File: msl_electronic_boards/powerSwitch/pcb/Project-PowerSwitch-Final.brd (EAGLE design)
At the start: 65.3 x 99.7 mm, 130 parts, among them IC10 BTS6133, IC11 BTS6133, IC12 BTS6133, IC15 BTS6133, IC3 LM2574M-5.0, IC4 BTS555E3146, IC7 MAX202, Q1 16Mhz, T1 BC847, T2 BC849, T5 BC849, T6 BC849, T7 BC849

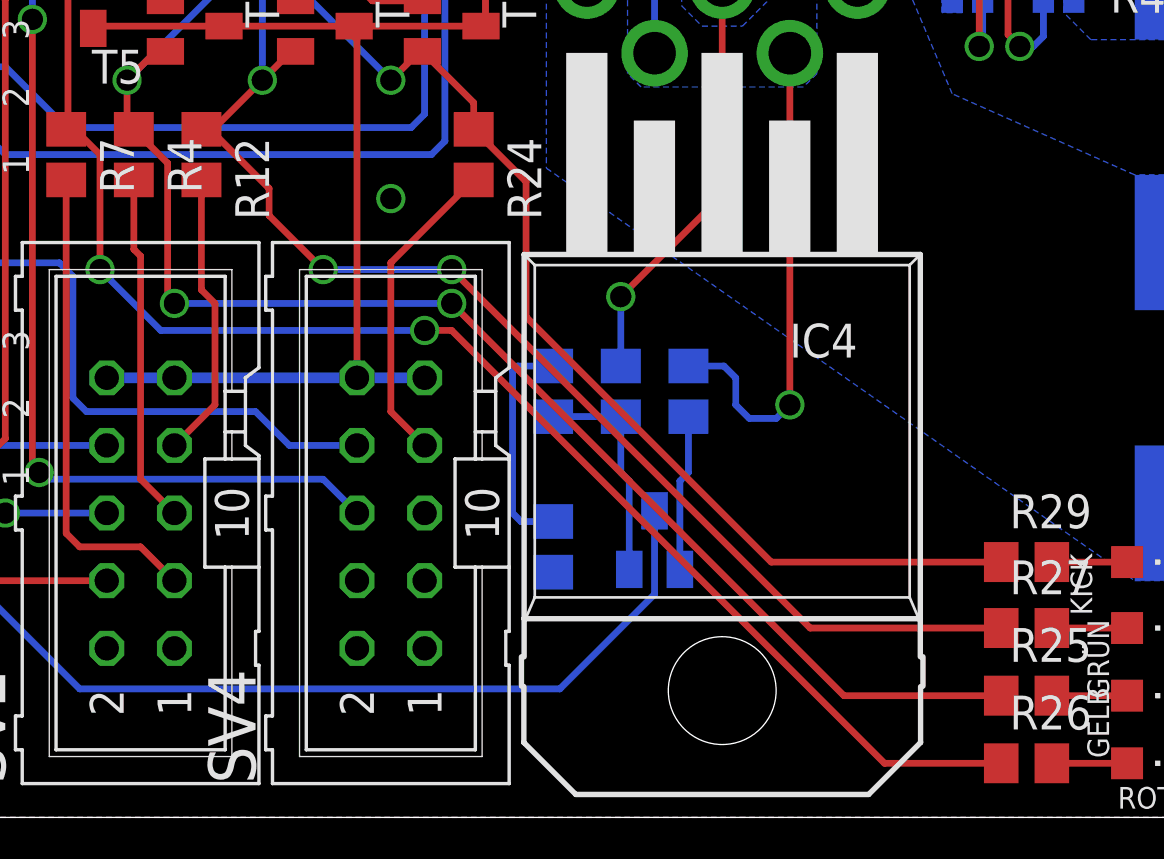
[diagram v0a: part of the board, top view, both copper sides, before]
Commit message: PCB PowerSwitch
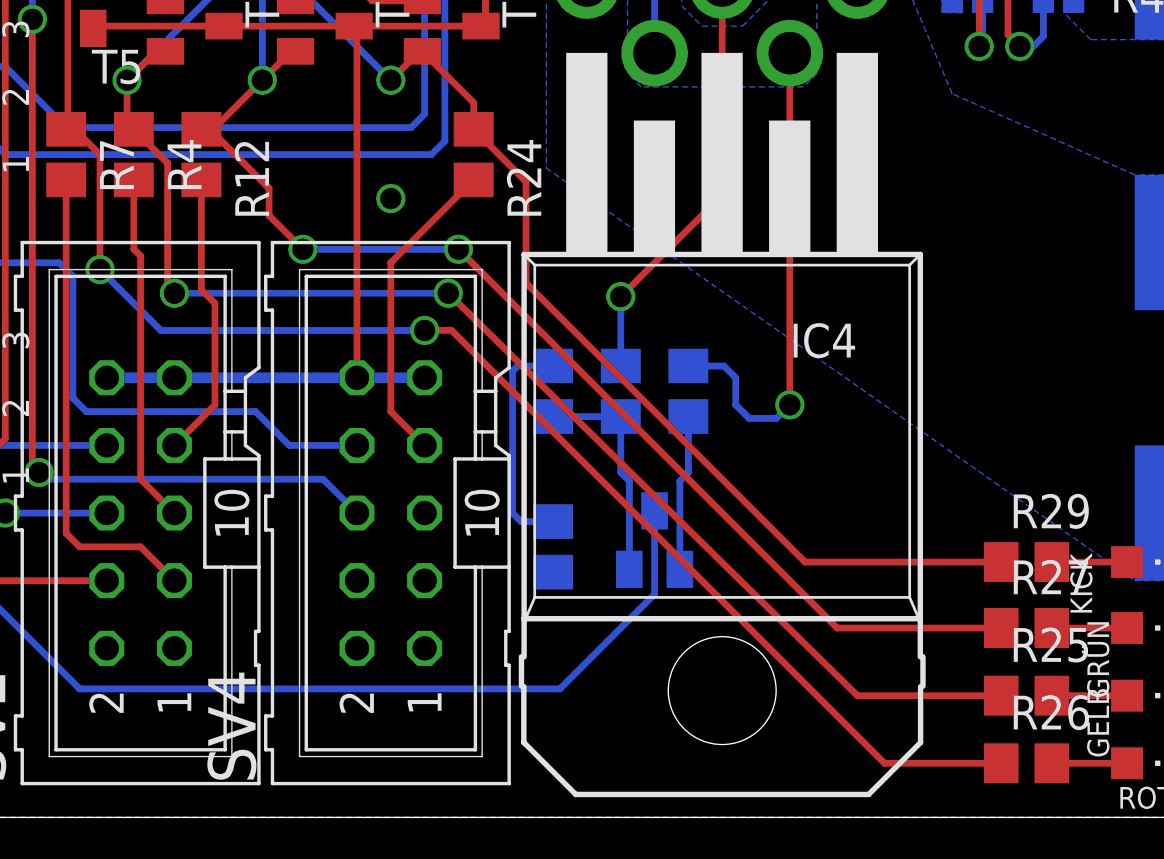
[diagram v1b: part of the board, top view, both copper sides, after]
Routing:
- net ICLED_KICK: track 89.0 -> 88.3 mm
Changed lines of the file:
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@@
 <wire x1="24.3" y1="28.768" x2="26.2255" y2="26.8425" width="0.254" layer="1"/>
 <wire x1="26.2255" y1="26.8425" x2="26.2255" y2="25.842" width="0.254" layer="1"/>
-<wire x1="46.04" y1="9.5885" x2="37.4015" y2="9.5885" width="0.254" layer="1"/>
-<wire x1="37.4015" y1="9.5885" x2="28.194" y2="18.796" width="0.254" layer="1"/>
-<wire x1="28.194" y1="18.796" x2="28.194" y2="23.8735" width="0.254" layer="1"/>
+<wire x1="46.04" y1="9.5885" x2="38.6715" y2="9.5885" width="0.254" layer="1"/>
+<wire x1="38.6715" y1="9.5885" x2="28.194" y2="20.066" width="0.254" layer="1"/>
+<wire x1="28.194" y1="20.066" x2="28.194" y2="23.8735" width="0.254" layer="1"/>
 <wire x1="28.194" y1="23.8735" x2="26.2255" y2="25.842" width="0.254" layer="1"/>
 <wire x1="24.3" y1="28.768" x2="24.196" y2="28.768" width="0.254" layer="1"/>
@@
 <contactref element="R27" pad="1"/>
 <contactref element="U$2" pad="28"/>
-<wire x1="46.04" y1="7.112" x2="38.862" y2="7.112" width="0.254" layer="1"/>
-<wire x1="38.862" y1="7.112" x2="25.4" y2="20.574" width="0.254" layer="1"/>
-<via x="25.4" y="20.574" extent="1-16" drill="0.8"/>
-<wire x1="25.4" y1="20.574" x2="20.574" y2="20.574" width="0.254" layer="16"/>
-<via x="20.574" y="20.574" extent="1-16" drill="0.8"/>
+<wire x1="46.04" y1="7.112" x2="39.878" y2="7.112" width="0.254" layer="1"/>
+<wire x1="39.878" y1="7.112" x2="25.654" y2="21.336" width="0.254" layer="1"/>
+<via x="25.654" y="21.336" extent="1-16" drill="0.8"/>
+<wire x1="25.654" y1="21.336" x2="19.812" y2="21.336" width="0.254" layer="16"/>
+<via x="19.812" y="21.336" extent="1-16" drill="0.8"/>
 <wire x1="19.5375" y1="28.6815" x2="19.2835" y2="28.6815" width="0.254" layer="1"/>
 <wire x1="18.288" y1="27.686" x2="16.51" y2="25.908" width="0.254" layer="1"/>
@@
 <wire x1="19.05" y1="64.008" x2="20.574" y2="65.532" width="0.254" layer="1"/>
 <via x="20.574" y="65.532" extent="1-16" drill="0.8"/>
-<wire x1="20.574" y1="20.574" x2="18.542" y2="22.606" width="0.254" layer="1"/>
+<wire x1="19.812" y1="21.336" x2="18.542" y2="22.606" width="0.254" layer="1"/>
 <wire x1="18.542" y1="22.606" x2="18.542" y2="23.622" width="0.254" layer="1"/>
 <wire x1="18.542" y1="23.622" x2="16.322" y2="25.842" width="0.254" layer="1"/>
@@
 <contactref element="R25" pad="1"/>
 <contactref element="U$2" pad="30"/>
-<wire x1="46.04" y1="4.572" x2="40.132" y2="4.572" width="0.254" layer="1"/>
-<wire x1="40.132" y1="4.572" x2="25.4" y2="19.304" width="0.254" layer="1"/>
-<via x="25.4" y="19.304" extent="1-16" drill="0.8"/>
-<wire x1="25.4" y1="19.304" x2="14.986" y2="19.304" width="0.254" layer="16"/>
-<via x="14.986" y="19.304" extent="1-16" drill="0.8"/>
-<wire x1="14.986" y1="19.304" x2="14.732" y2="19.558" width="0.254" layer="1"/>
-<wire x1="14.732" y1="19.558" x2="14.732" y2="24.572" width="0.254" layer="1"/>
+<wire x1="46.04" y1="4.572" x2="40.64" y2="4.572" width="0.254" layer="1"/>
+<wire x1="40.64" y1="4.572" x2="25.273" y2="19.685" width="0.254" layer="1"/>
+<via x="25.273" y="19.685" extent="1-16" drill="0.8"/>
+<wire x1="25.273" y1="19.685" x2="14.986" y2="19.685" width="0.254" layer="16"/>
+<via x="14.986" y="19.685" extent="1-16" drill="0.8"/>
+<wire x1="14.986" y1="19.685" x2="14.732" y2="19.939" width="0.254" layer="1"/>
+<wire x1="14.732" y1="19.939" x2="14.732" y2="24.572" width="0.254" layer="1"/>
 <wire x1="14.732" y1="24.572" x2="13.462" y2="25.842" width="0.254" layer="1"/>
 <wire x1="13.208" y1="27.686" x2="13.208" y2="26.096" width="0.254" layer="1"/>
